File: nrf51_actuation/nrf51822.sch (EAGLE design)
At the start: 25 parts, among them T1 MMUN2238

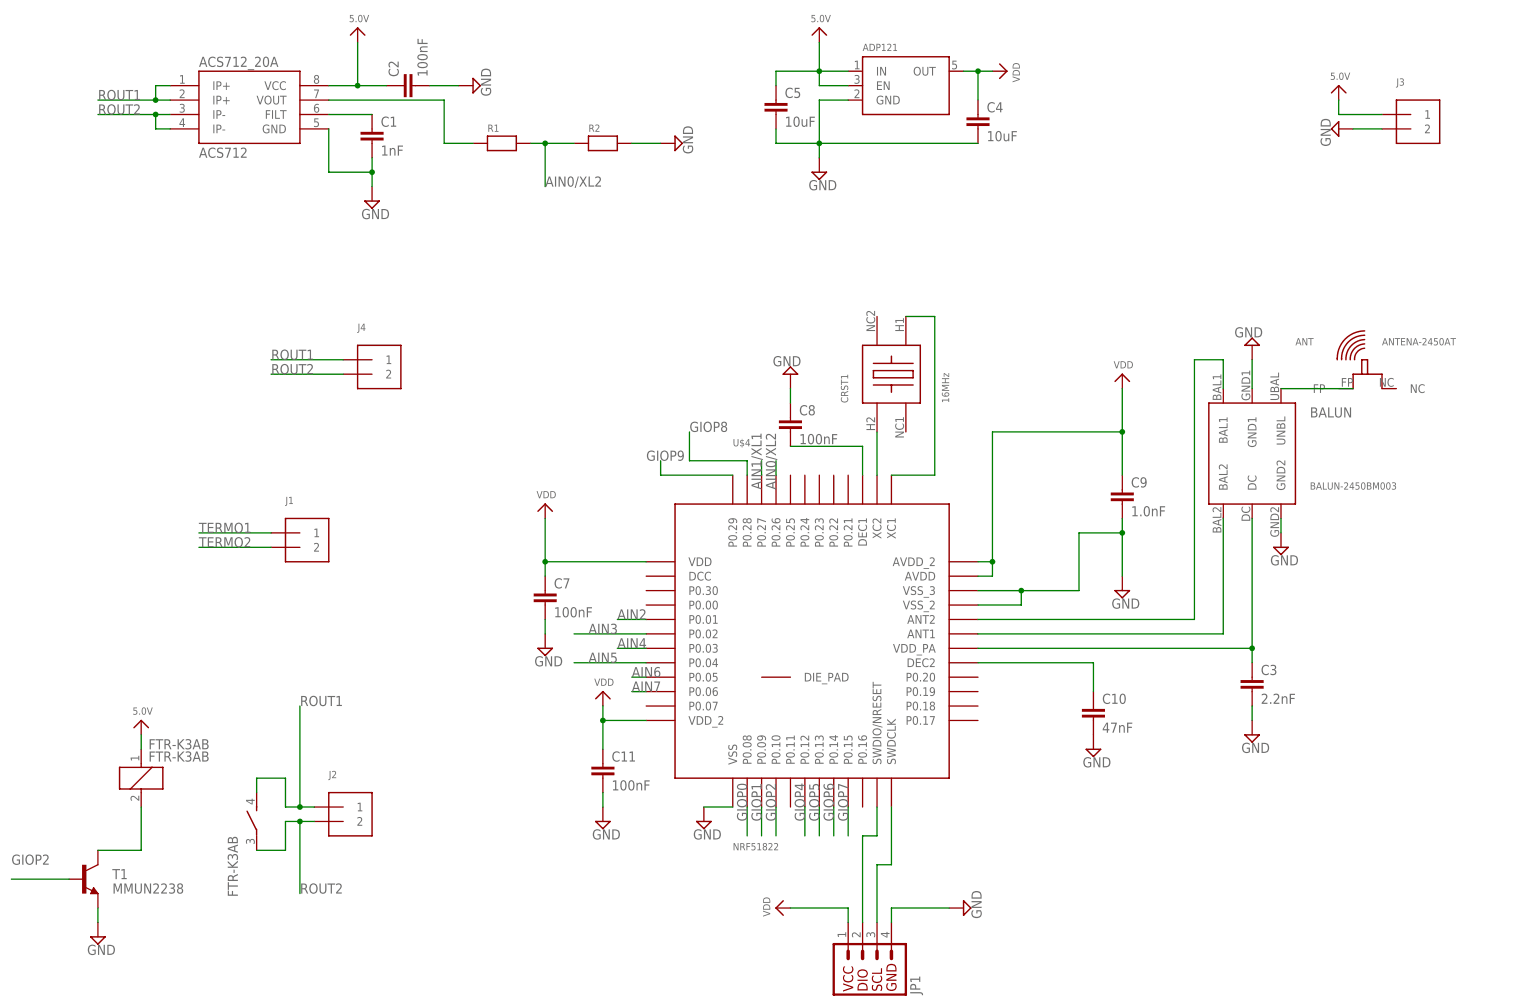
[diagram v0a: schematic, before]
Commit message: Done with routing.. should be more or less done
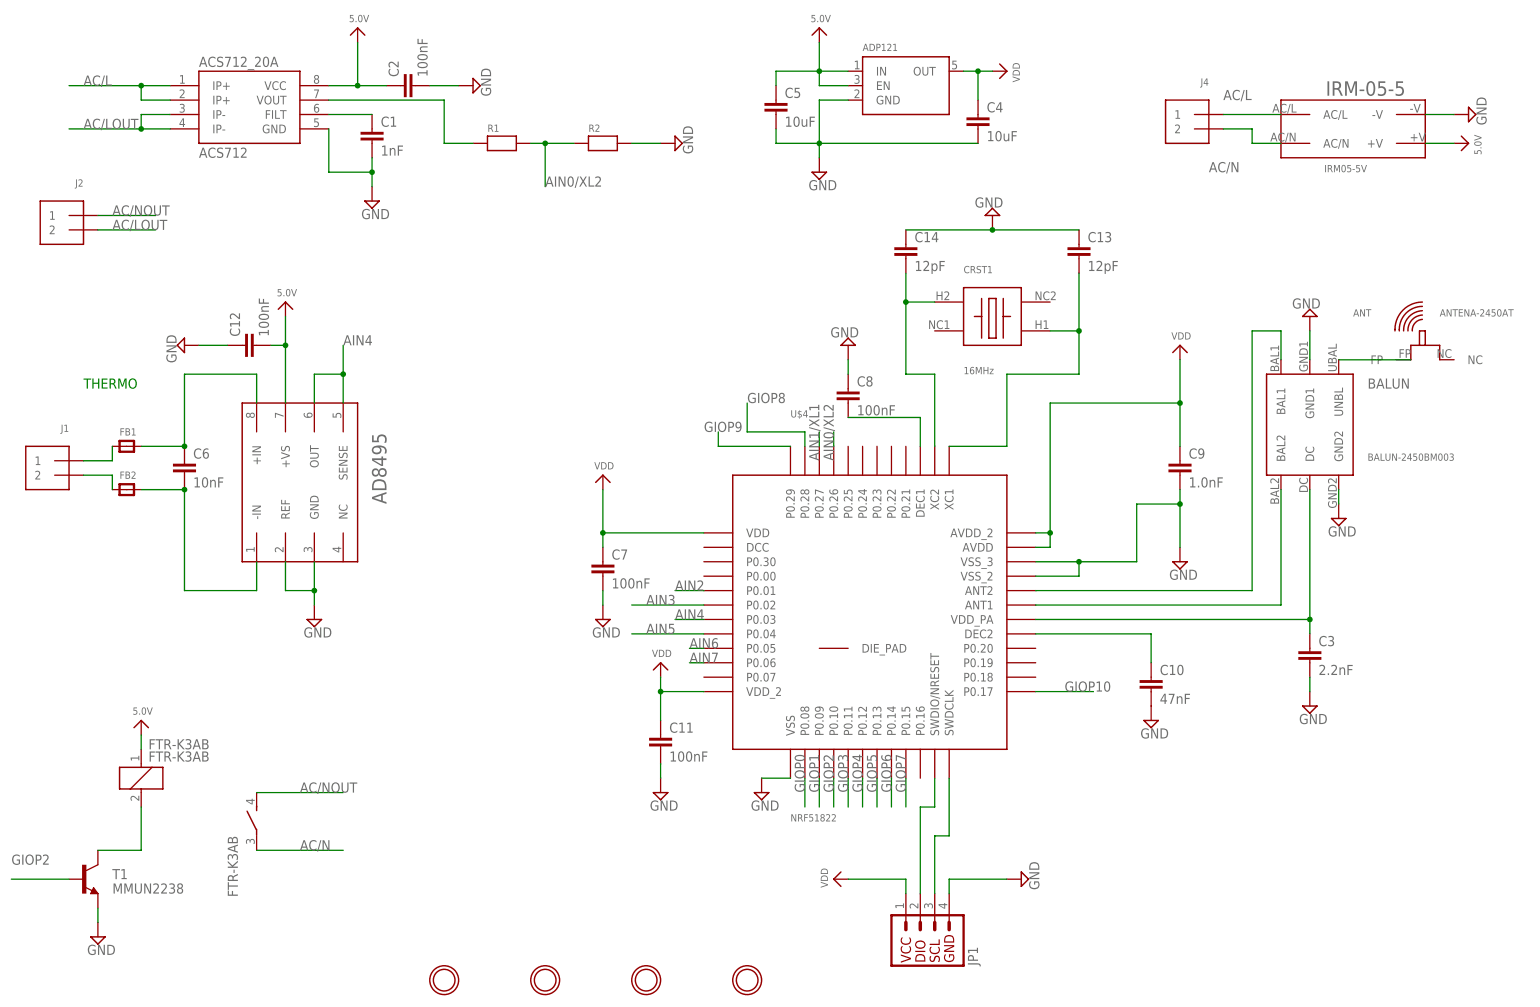
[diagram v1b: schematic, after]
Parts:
- removed J3: (no value), microbuilder:TERMBLOCK_1X2
- added AD8495: AD8495, NordicSemi:AD8495
- added C12: 100nF, rcl:C-EUC0805
- added C13, C14: 12pF, rcl:C-EUC0805
- added C6: 10nF, rcl:C-EUC0805
- added FB1, FB2: (no value), microbuilder:FERRITE0805
- added IRM-05-5: IRM05-5V, NordicSemi:IRM05-5V
- added U$1, U$13, U$14, U$7: MOUNTINGHOLE2.5, microbuilder:MOUNTINGHOLE2.5
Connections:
- removed net ROUT1: ACS712_20A.IP+@1, ACS712_20A.IP+@2, FTR-K3ABG$1.4, J2.1, J4.1
- removed net ROUT2: ACS712_20A.IP-@3, ACS712_20A.IP-@4, FTR-K3ABG$1.3, J2.2, J4.2
- removed net TERMO1: J1.1
- removed net TERMO2: J1.2
- new net AC/L: ACS712_20A.IP+@1, ACS712_20A.IP+@2, IRM-05-5.AC/L, J4.1
- new net AC/LOUT: ACS712_20A.IP-@3, ACS712_20A.IP-@4, J2.2
- new net AC/N: FTR-K3ABG$1.3, IRM-05-5.AC/N, J4.2
- new net AC/NOUT: FTR-K3ABG$1.4, J2.1
- new net GIOP10: U$4.P0.17
- new net GIOP3: U$4.P0.11
- new net N$16: AD8495.-IN, C6.2, FB2.P$2
- new net N$17: FB2.P$1, J1.2
- new net N$8: FB1.P$1, J1.1
- new net N$9: AD8495.+IN, C6.1, FB1.P$2
- net 5.0V: now also AD8495.+VS, C12.2, IRM-05-5.+V; no longer J3.1
- net AIN4: now also AD8495.OUT, AD8495.SENSE
- net GND: now also AD8495.GND, AD8495.REF, C12.1, C13.1, C14.1, IRM-05-5.-V; no longer J3.2
- net N$1: now also C14.2, CRST1.H2, U$4.XC2; no longer CRST1.H1, U$4.XC1
- net N$2: now also C13.2, CRST1.H1, U$4.XC1; no longer CRST1.H2, U$4.XC2
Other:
- note added: "THERMO"
- moved on the sheet: ANT, BALUN, C10, C11, C3, C7, C8, C9, CRST1, J1, J2, J4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
